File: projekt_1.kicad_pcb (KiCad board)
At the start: 2 copper layers, 99.6 x 91.3 mm, 38 parts, among them J1 Screw_DS18_Terminal_01x03, J3 Czajnik_plug, J4 Conn_01x15_Female, J5 Conn_01x15_Female, J6 Screw_230v_Terminal_01x03, Q1 BSS138, Q2 BTA16-600C, U2 MOC3041M

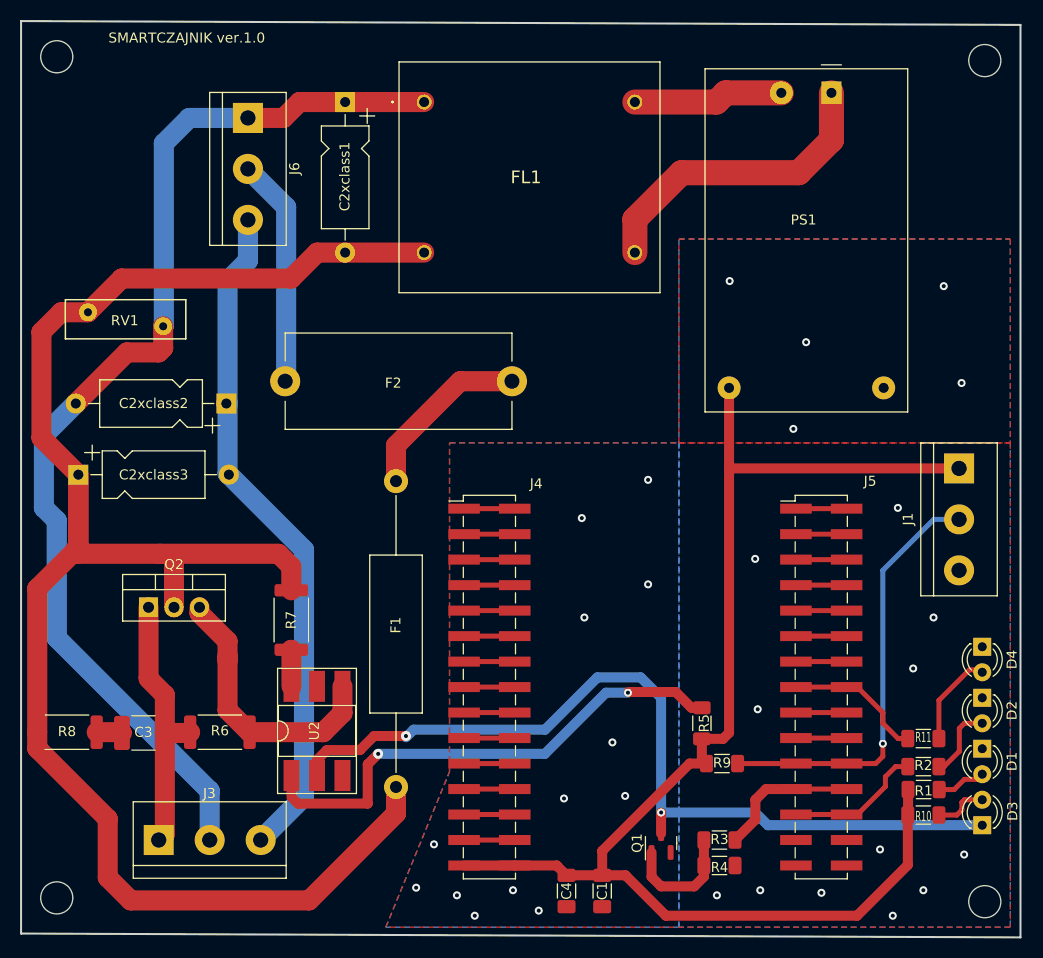
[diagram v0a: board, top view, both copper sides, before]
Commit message: Add files via upload
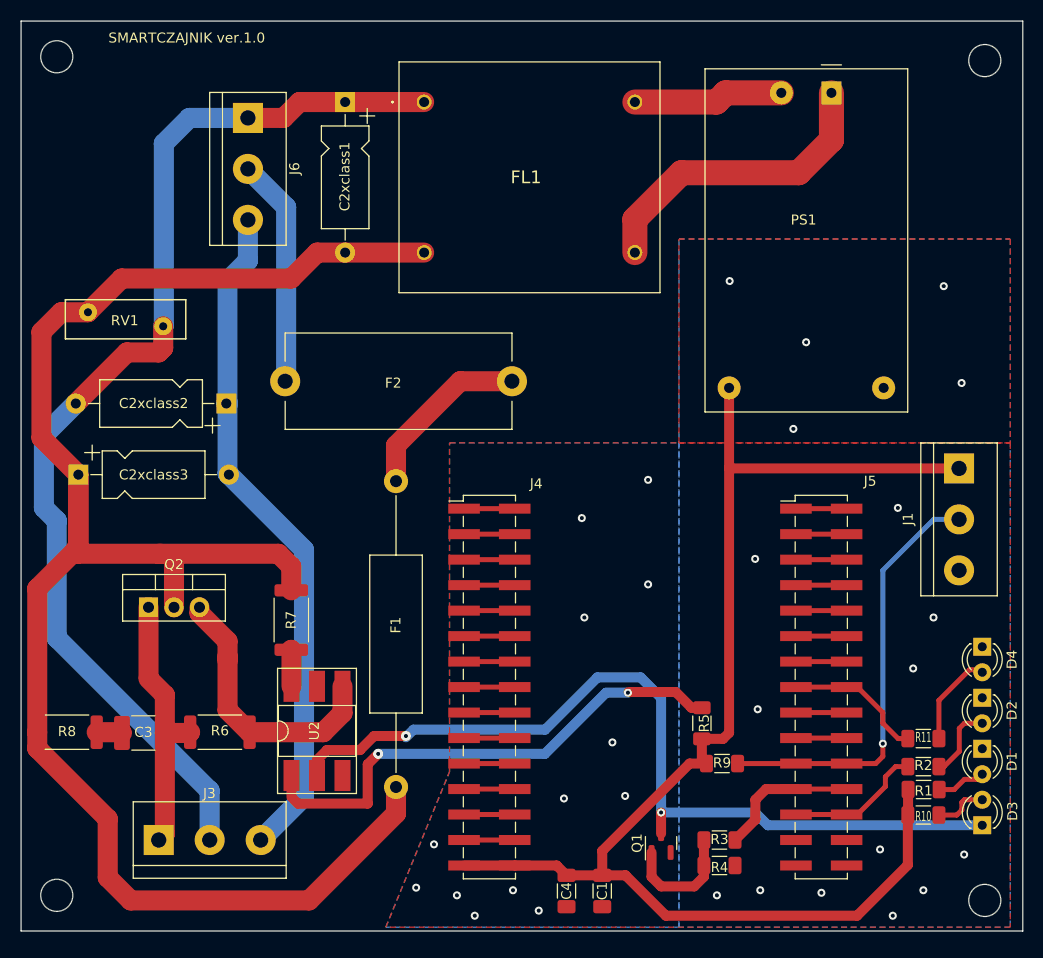
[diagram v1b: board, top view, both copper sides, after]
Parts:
- moved H4 0.25 mm to (26.9, 101.0)
- moved H3 0.13 mm to (119.4, 101.5)
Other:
- board size 99.6 x 91.3 mm -> 99.8 x 90.7 mm
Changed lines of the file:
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@@
       (drillshape 0)
       (scaleselection 1)
-      (outputdirectory "../../../Desktop/smartczajnik/pdfy_gerbery/")
+      (outputdirectory "gerber/")
     )
   )
@@
   )
   (footprint "MountingHole:MountingHole_3.2mm_M3" (layer "F.Cu")
-    (at 26.8986 101.2192)
+    (at 26.8986 100.9652)
     (descr "Mounting Hole 3.2mm, no annular, M3")
     (tags "mounting hole 3.2mm no annular m3")
@@
   )
   (footprint "MountingHole:MountingHole_3.2mm_M3" (layer "F.Cu")
-    (at 119.38 101.6)
+    (at 119.38 101.4732)
     (descr "Mounting Hole 3.2mm, no annular, M3")
     (tags "mounting hole 3.2mm no annular m3")
@@
     )
   )
-  (gr_line (start 23.3426 104.7752) (end 23.3426 13.8432) (layer "Edge.Cuts") (width 0.2))
-  (gr_line (start 122.936 105.156) (end 23.3426 104.7752) (layer "Edge.Cuts") (width 0.2))
-  (gr_line (start 23.3426 13.8432) (end 122.936 14.224) (layer "Edge.Cuts") (width 0.2))
-  (gr_line (start 122.936 14.224) (end 122.936 105.156) (layer "Edge.Cuts") (width 0.2))
+  (gr_rect (start 123.1646 13.8432) (end 23.3426 104.5212) (layer "Edge.Cuts") (width 0.1) (fill none))
   (gr_text "SMARTCZAJNIK ver.1.0" (at 39.8526 15.5196) (layer "F.SilkS")
     (effects (font (size 1 1) (thickness 0.15)))
